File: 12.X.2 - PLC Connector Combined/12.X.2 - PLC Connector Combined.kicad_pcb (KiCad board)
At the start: 2 copper layers, 61.5 x 72.3 mm, 73 parts, among them J201 Conn_01x01_PAD, J202 Conn_01x01_PAD, J203 Conn_01x01_PAD, J204 Conn_01x01_PAD, J205 Conn_01x01_PAD, J206 Conn_01x01_PAD, J207 Conn_01x01_PAD, J208 Conn_01x01_PAD, J209 Conn_01x01_PAD, J210 Conn_01x01_PAD, J211 Conn_01x01_PAD, J212 Conn_01x01_PAD, J213 Conn_01x01_PAD, J214 Conn_01x01_PAD, J215 Conn_01x01_PAD, J216 Conn_01x01_PAD, J217 Conn_01x01_PAD, J218 Conn_01x01_PAD, J219 Conn_01x01_PAD, J220 Conn_01x01_PAD, J221 Dorabo-DB128L_5_08_2P_BKS, J222 Dorabo-DB128L_5_08_2P_BKS, J223 Dorabo-DB128L_5_08_2P_BKS, J224 Dorabo-DB128L_5_08_2P_BKS, J225 Dorabo-DB128L_5_08_2P_BKS, J226 B04B-XASK-1, J301 Conn_01x01_PAD, J302 Conn_01x01_PAD, J303 Conn_01x01_PAD, J304 Conn_01x01_PAD, J305 Conn_01x01_PAD, J306 Conn_01x01_PAD, J307 Conn_01x01_PAD, J308 Conn_01x01_PAD, J309 Conn_01x01_PAD, J310 Conn_01x01_PAD, J311 Conn_01x01_PAD, J312 Conn_01x01_PAD, J313 Conn_01x01_PAD, J314 Conn_01x01_PAD, J315 Conn_01x01_PAD, J316 Conn_01x01_PAD, J317 DB128L-5.08-2P-BK-S, J318 DB128L-5.08-3P-BK-S, J319 DB128L-5.08-2P-BK-S, J320 DB128L-5.08-2P-BK-S, J321 B04B-XASK-1

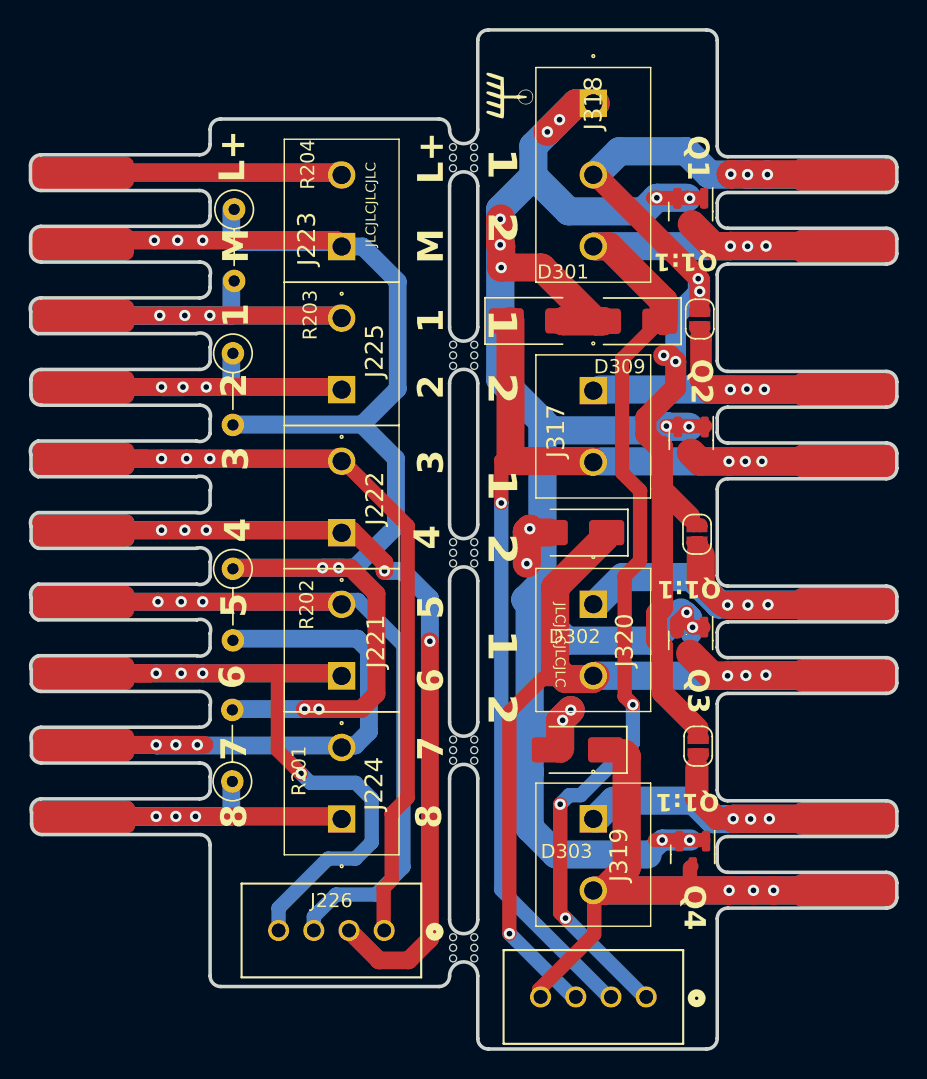
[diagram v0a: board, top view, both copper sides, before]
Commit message: updatd board outline
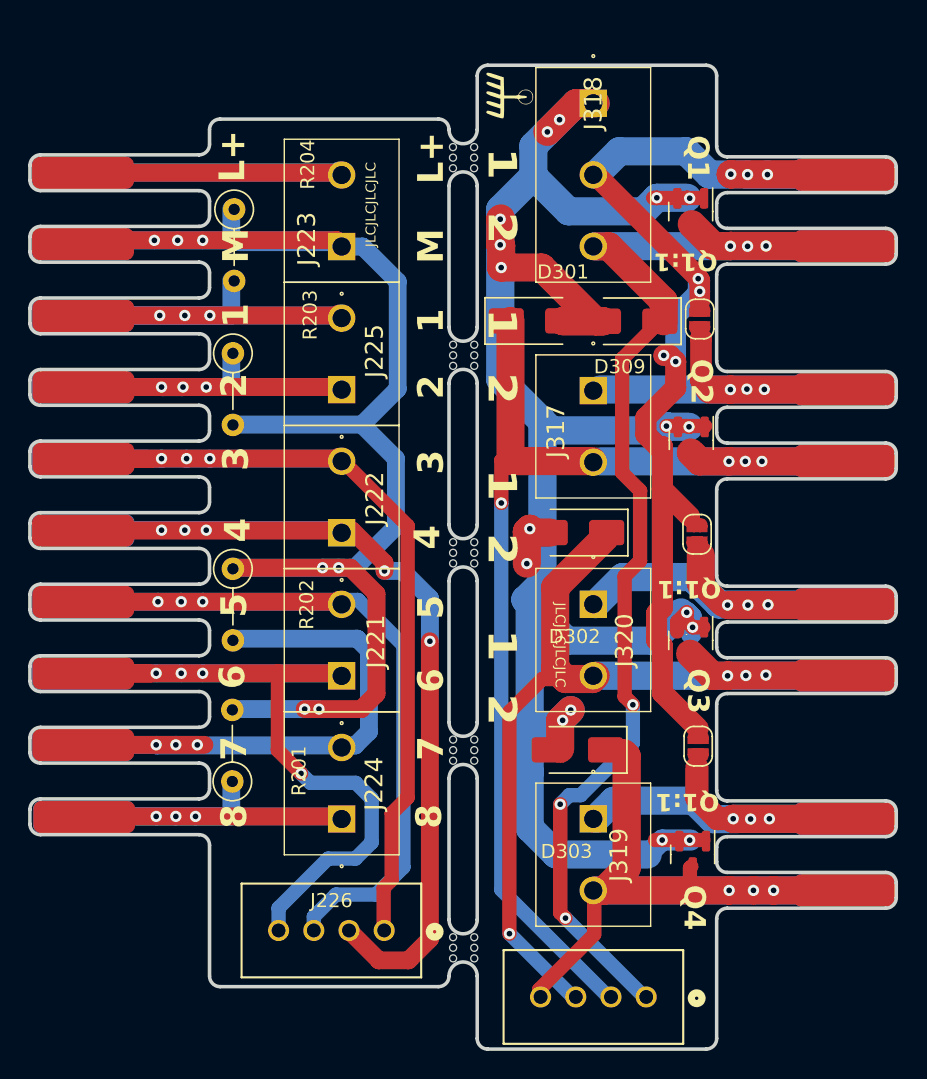
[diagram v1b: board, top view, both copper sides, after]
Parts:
- moved G*** 2.53 mm to (115.9, 67.1)
- moved G*** 2.32 mm to (105.8, 66.7)
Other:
- board size 61.5 x 72.3 mm -> 61.5 x 69.8 mm
